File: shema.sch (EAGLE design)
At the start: 14 parts

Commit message: добавила файлы
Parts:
- removed U$10: INDUCTOR, 1_NDUCTORS:INDUCTOR
- removed U$12: TRANSISTORN, 1_TRANSISTOR (2):TRANSISTORN
- removed U$14, U$2, U$3: RESISTOR0603, 1_RESISTOR:RESISTOR0603
- removed U$4, U$5: LED, 1_LED:LED
- removed U$8: B560C-13-F, 1_DIOD:B560C-13-F
- removed U$9: CAPACITOR, 1_RESISTOR:CAPACITOR
- added C0: 22uF, 1_RESISTOR:CAPACITOR
- added D1: B560C-13-F, 1_DIOD:B560C-13-F
- added D3, D4: LED, 1_LED:LED
- added L1: INDUCTOR, 1_NDUCTORS:INDUCTOR
- added M1: TRANSISTORN, 1_TRANSISTOR (2):TRANSISTORN
- added R1, R2, R3: RESISTOR0603, 1_RESISTOR:RESISTOR0603
- C1: value CAPACITOR -> 22uF
- renumbered U$1 to C1, U$11 to D2, U$6 to RCS, VT1 to M2
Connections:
- net 8.4V: now also C0.1, D1.C; no longer U$8.C, U$9.1
- net GND: now also C0.2, D4.C, M1.S; no longer U$12.S, U$5.C, U$9.2
- net N$1: now also D4.A, R2.P$1; no longer U$3.P$1, U$5.A
- net N$11: now also D3.C, R2.P$2; no longer U$3.P$2, U$4.C
- net N$12: now also D3.A, R1.P$1; no longer U$2.P$1, U$4.A
- net N$5: now also L1.1; no longer U$10.1
- net N$6: now also D1.A, L1.2, M1.D; no longer U$10.2, U$12.D, U$8.A
- net N$8: now also R3.P$2; no longer U$14.P$2
- net N$9: now also M1.G, R3.P$1; no longer U$12.G, U$14.P$1
- net V_IN: now also R1.P$2; no longer U$2.P$2

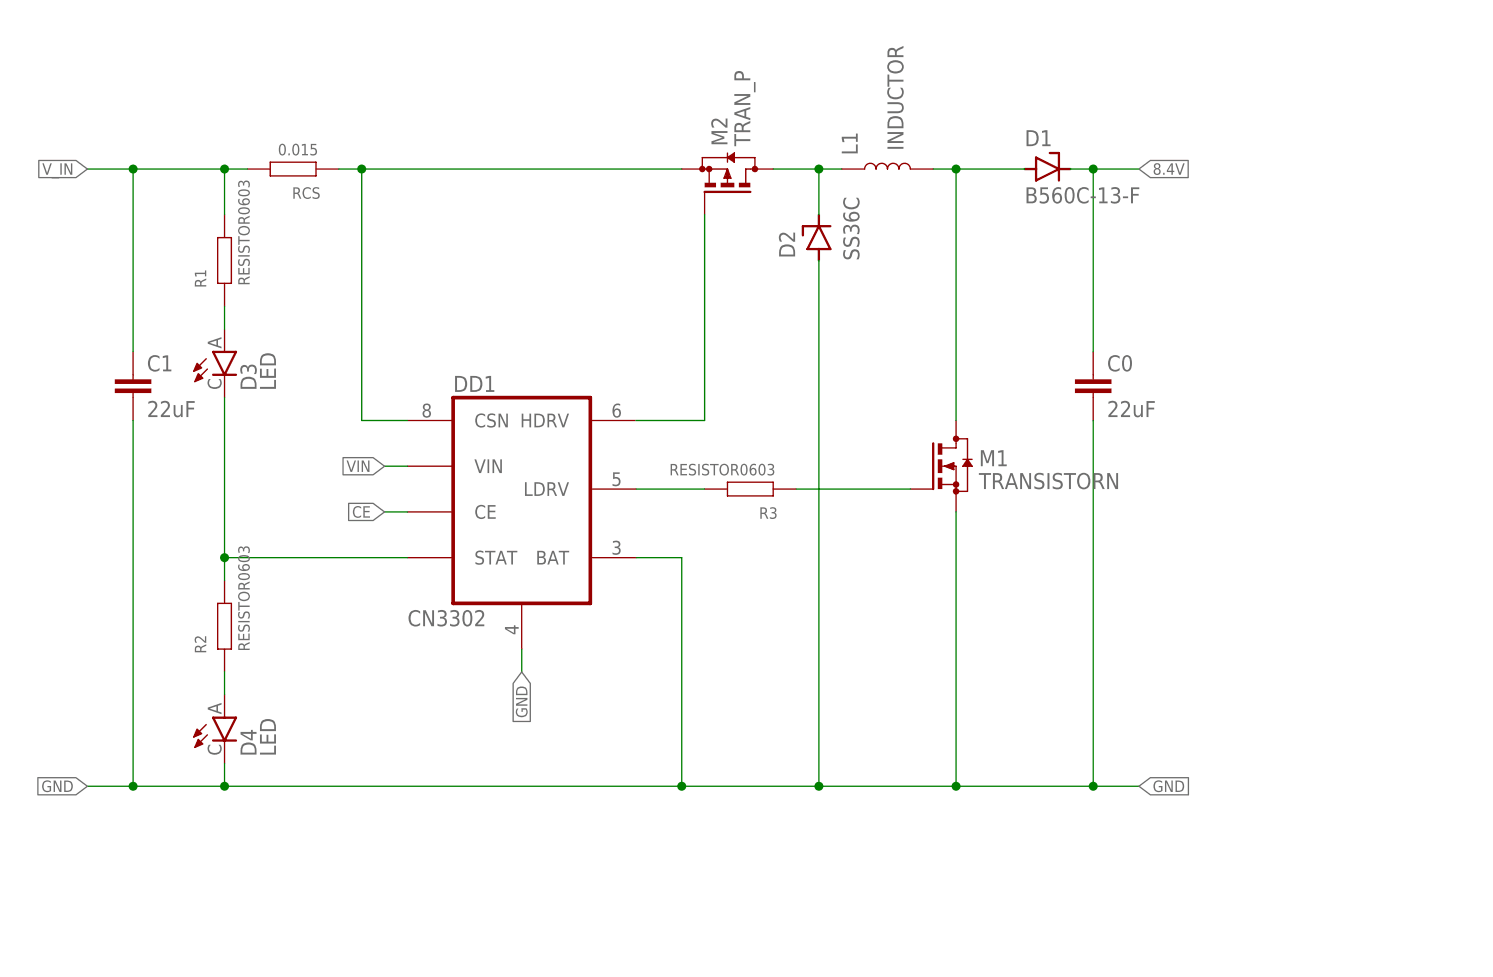
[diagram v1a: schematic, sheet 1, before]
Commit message: файлы изменение
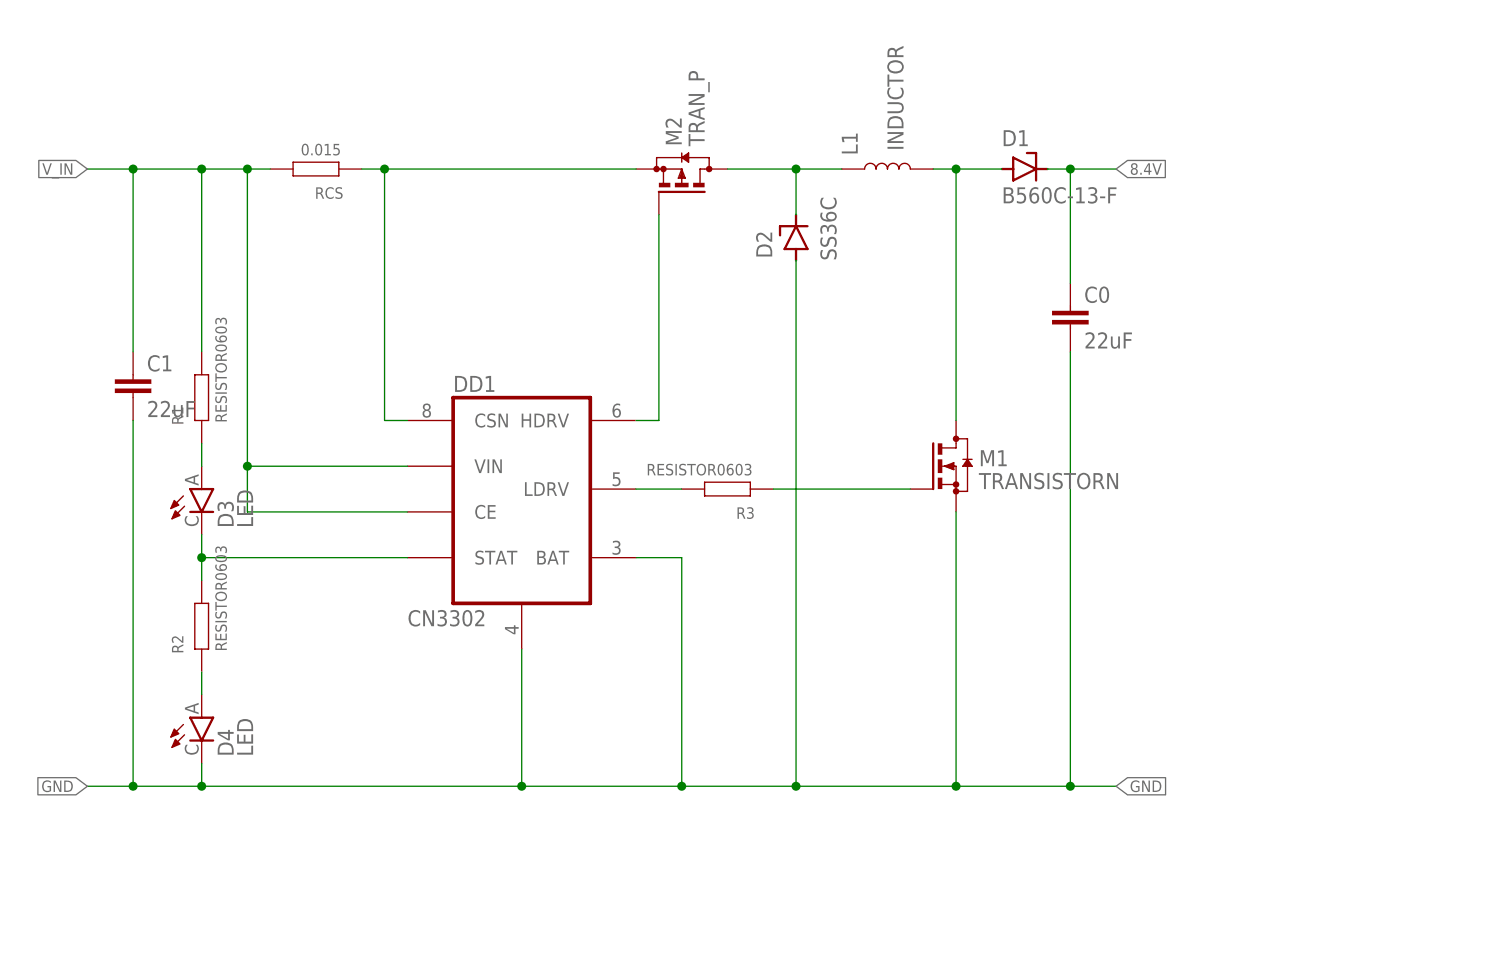
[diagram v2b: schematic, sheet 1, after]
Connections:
- removed net CE: DD1.CE
- removed net VIN: DD1.VIN
- net V_IN: now also DD1.CE, DD1.VIN
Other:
- moved on the sheet: C0, D1, D2, D3, D4, M2, R1, R2, R3, RCS

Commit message: fix
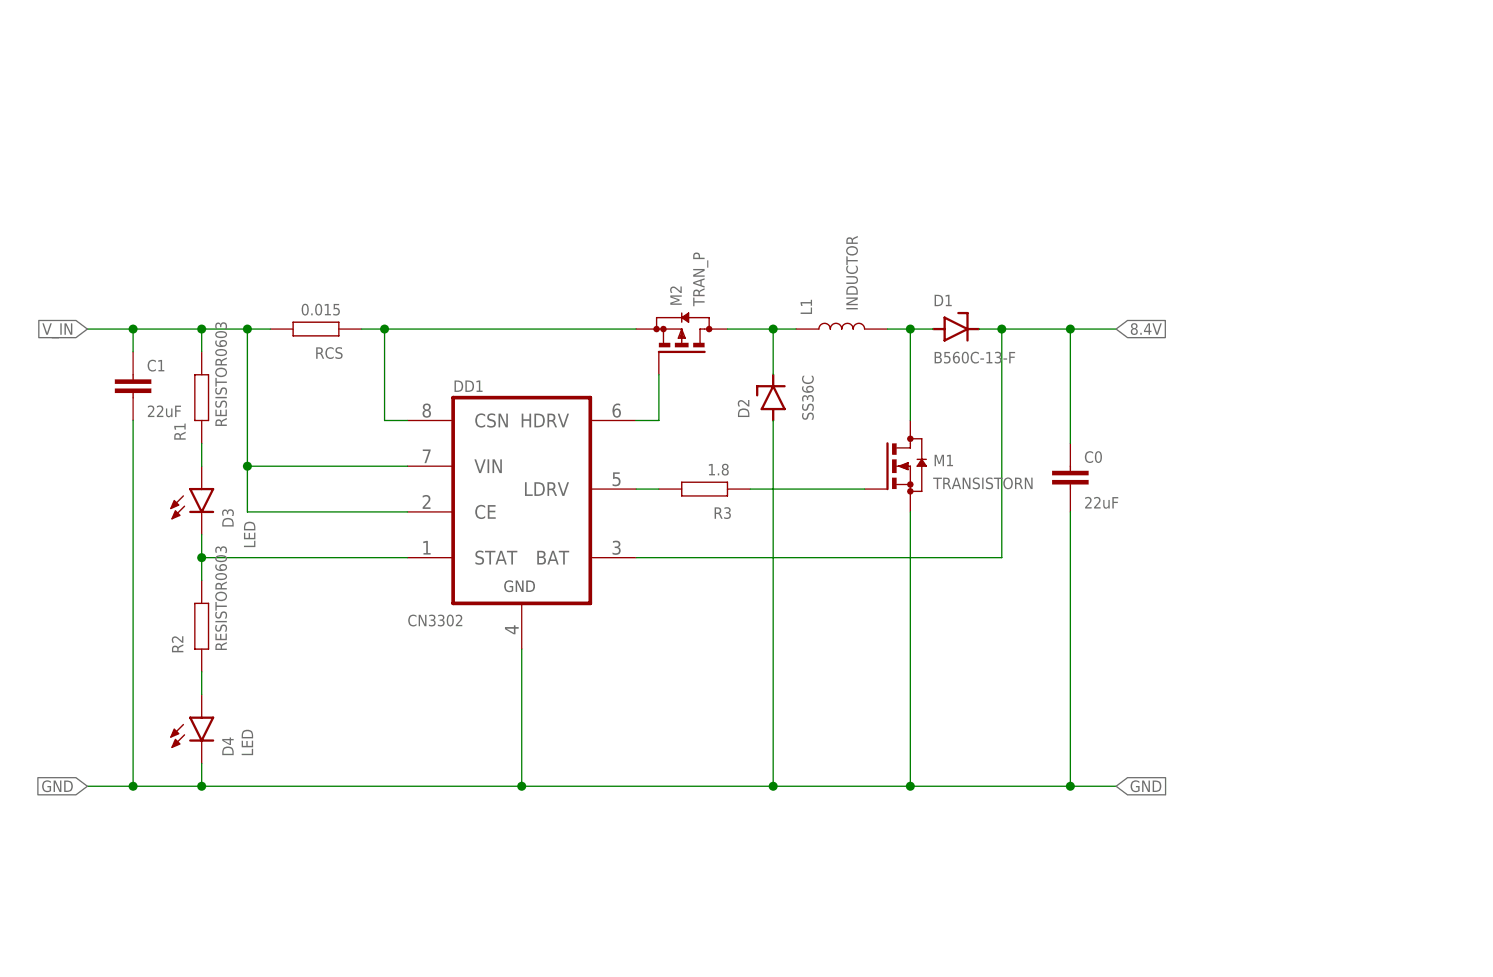
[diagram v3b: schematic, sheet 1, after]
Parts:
- R3: value RESISTOR0603 -> 1.8
- RCS: device 1_RESISTOR:RESISTOR0603 -> 1_RESISTOR:RESISTOR
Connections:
- net 8.4V: now also DD1.BAT
- net GND: no longer DD1.BAT
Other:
- moved on the sheet: C0, D1, D2, L1, M1, M2, R3, RCS

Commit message: файлы изменение
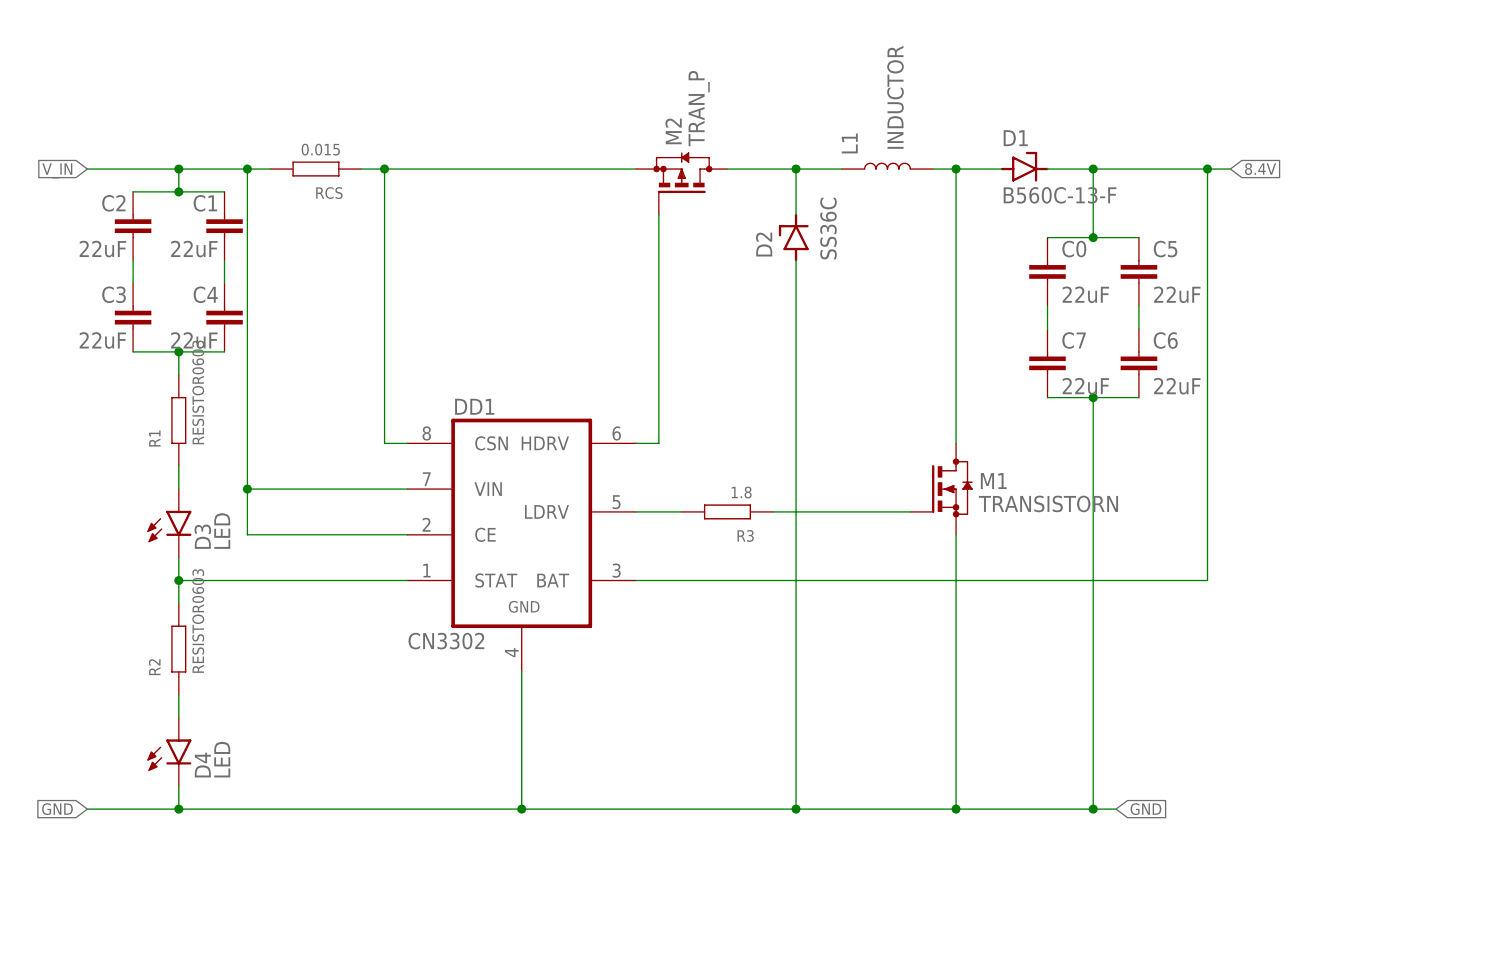
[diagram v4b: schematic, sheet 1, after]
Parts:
- added C2, C3, C4, C5, C6, C7: 22uF, 1_RESISTOR:CAPACITOR
- RCS: device 1_RESISTOR:RESISTOR -> 1_RESISTOR:RESISTOR0603
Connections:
- new net N$15: C5.2, C6.1
- new net N$16: C0.2, C7.1
- new net N$2: C2.2, C3.1
- new net N$3: C1.2, C4.1
- new net N$7: C3.2, C4.2, R1.P$2
- net 8.4V: now also C5.1
- net GND: now also C6.2, C7.2; no longer C0.2, C1.2
- net V_IN: now also C2.1; no longer R1.P$2
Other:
- moved on the sheet: C0, C1, D1, D2, D3, D4, DD1, L1, M1, M2, R1, R2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
